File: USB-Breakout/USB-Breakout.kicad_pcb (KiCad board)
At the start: 2 copper layers, 25 x 25 mm, 16 parts, among them J1 Conn_02x07_Odd_Even, J2 12401951E412A, Q1 IRLZ44N, Q2 IRF4905, U1 FUSB302BMPX

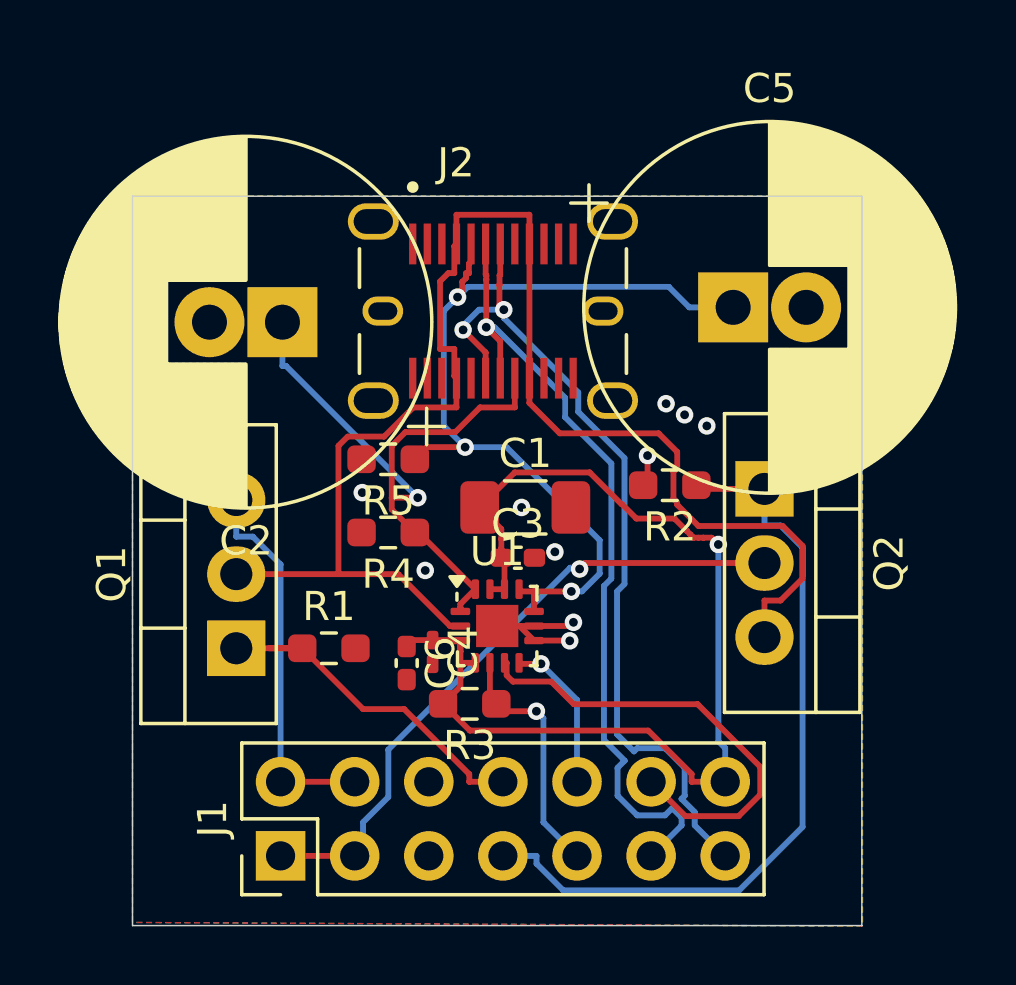
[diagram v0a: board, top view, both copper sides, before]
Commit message: Update documentation and improve project structure for better usability
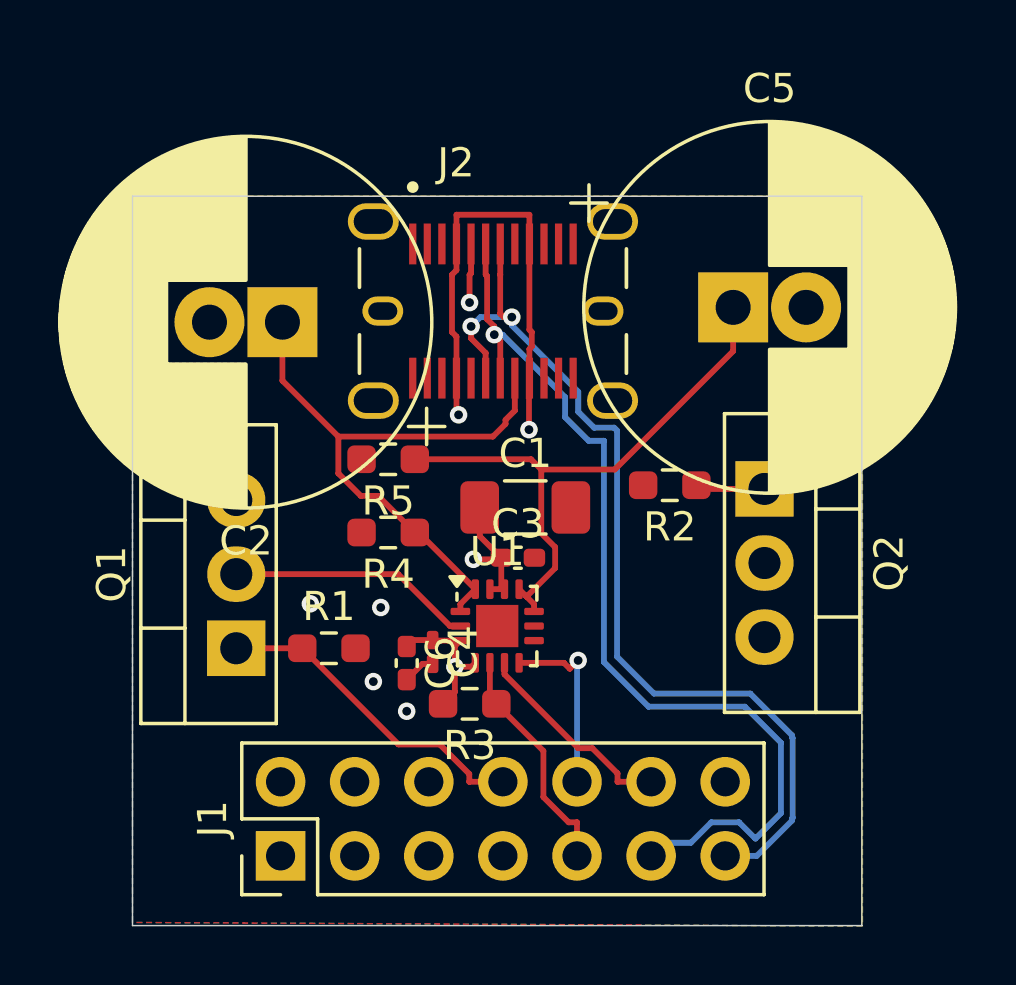
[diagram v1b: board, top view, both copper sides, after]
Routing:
- net +3.3V: track 38.7 -> 24.5 mm, vias 1 -> 2
- net +5V: track 22.3 -> 32.3 mm, vias 1 -> 0
- net /SCL: track 16.0 -> 7.11 mm
- net /D+: track 27.8 -> 33.2 mm
- net GND: track 6.44 -> 1.11 mm, vias 10 -> 4
- net /D-: track 29.0 -> 32.7 mm
- net /CC1: track 30.3 -> 32.7 mm, vias 3 -> 1
- net VBUS: track 50.4 -> 52.6 mm, vias 0 -> 2
- net /5_EN: track 26.7 -> 25.4 mm
- net /12_EN: track 12.3 -> 11.2 mm
- net /CC2: track 22.0 -> 20.9 mm, vias 1 -> 0
- net /SDA: track 5.32 -> 6.40 mm
- net /INT: track 8.61 -> 8.02 mm, vias 1 -> 0
- added copper zone on In1.Cu, net GND
- added copper zone on In2.Cu, net GND
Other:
- copper layers 2 -> 4
